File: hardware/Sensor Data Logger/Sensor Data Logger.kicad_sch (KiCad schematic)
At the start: 28 parts, among them J1 Conn_01x04_Male, J2 Conn_01x04_Male, J3 Conn_01x05_Male, J4 Conn_01x03_Male, SW1 SW_Push, SW2 SW_Push, SW3 SW_Push, U1 AMS1117-3.3, U2 ESP32-WROOM-32, U3 DS3231M

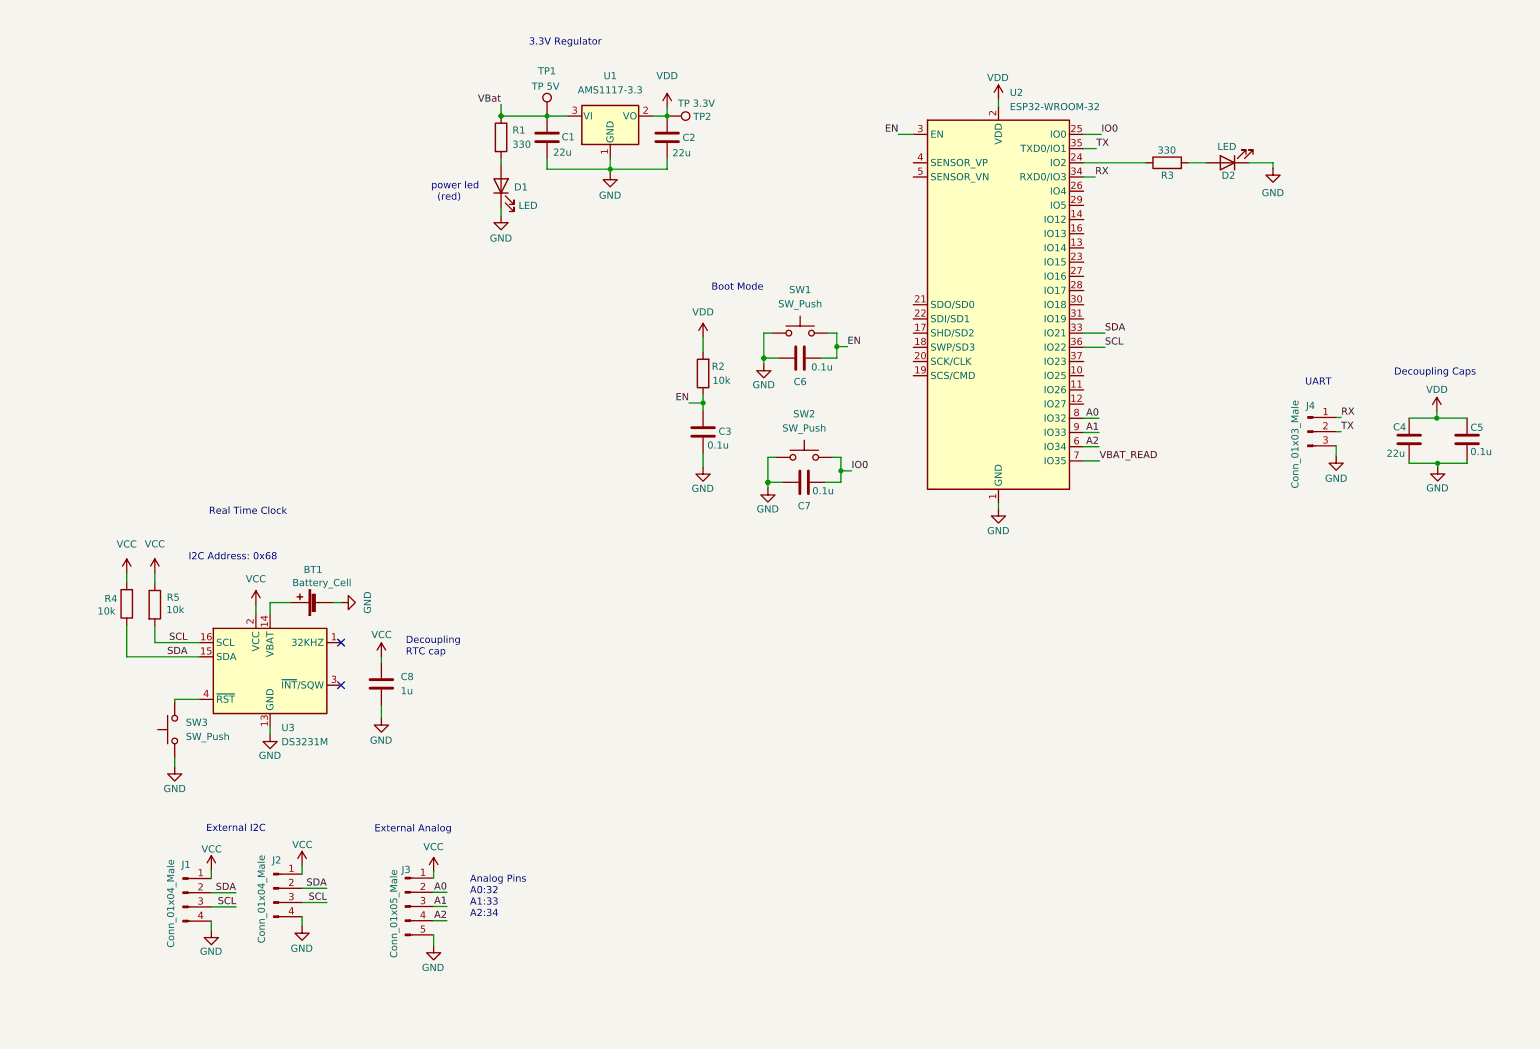
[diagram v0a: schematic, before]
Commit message: Latest schematic
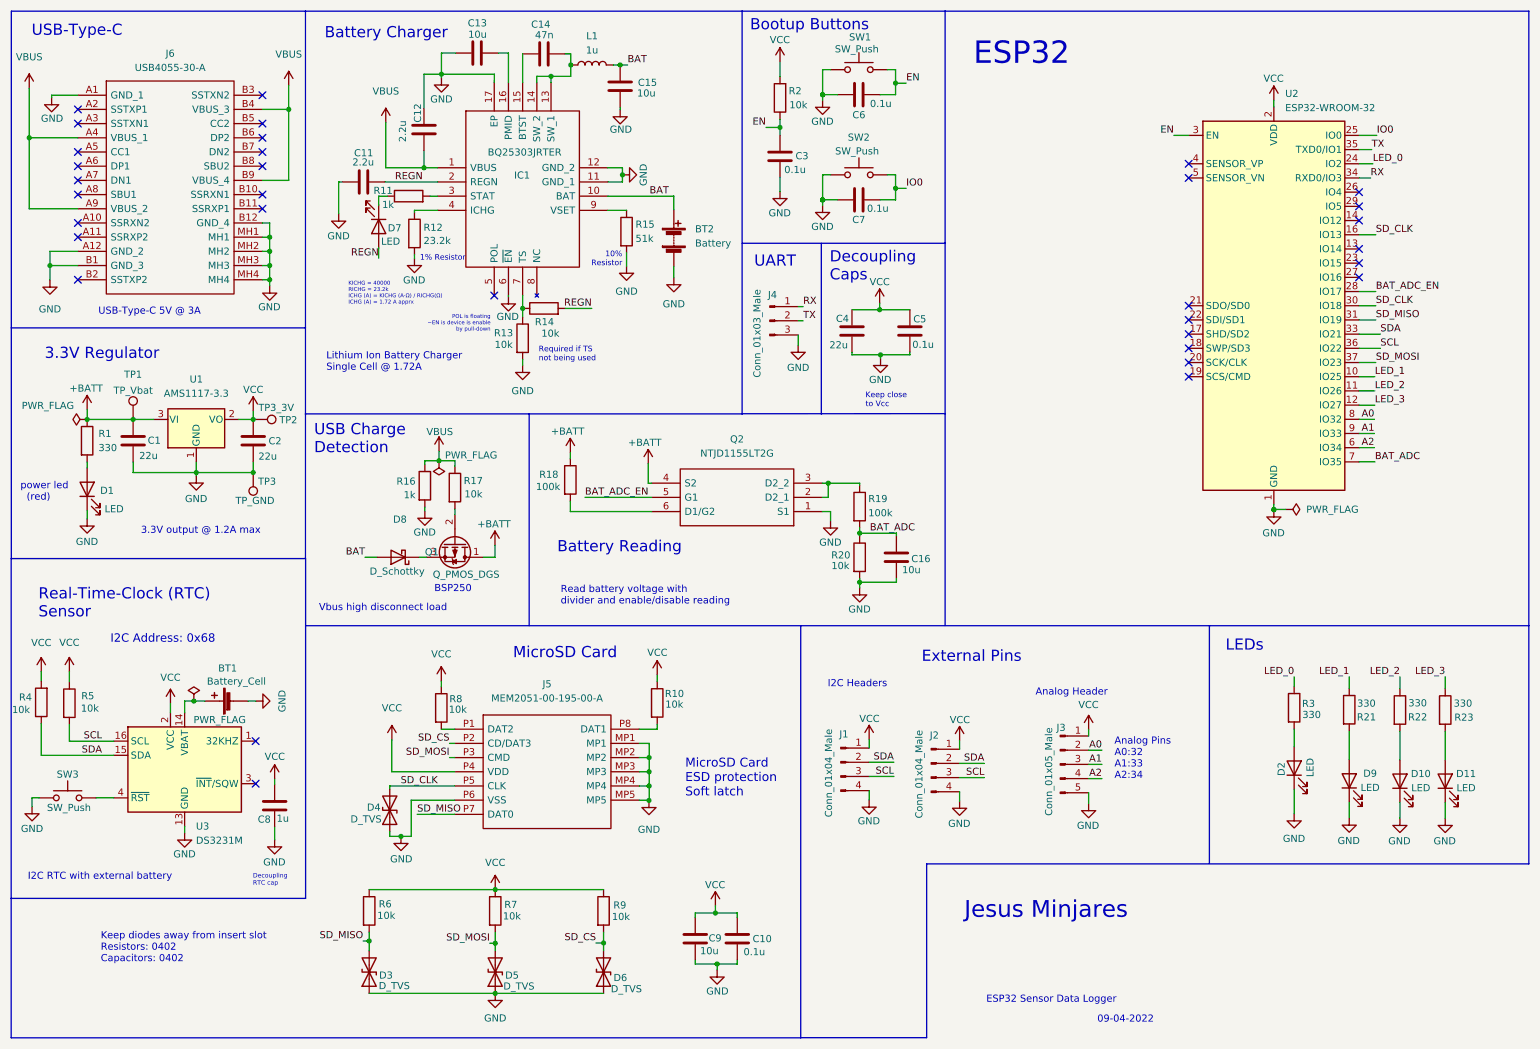
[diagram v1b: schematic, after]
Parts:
- added BT2: Battery, symbol Device:Battery
- added C10: 0.1u, symbol Device:C
- added C11, C12: 2.2u, symbol Device:C
- added C13, C15, C16, C9: 10u, symbol Device:C
- added C14: 47n, symbol Device:C
- added D10, D11, D7, D9: LED, symbol Device:LED
- added D3, D4, D5, D6: D_TVS, symbol Device:D_TVS
- added D8: D_Schottky, symbol Device:D_Schottky
- added IC1: BQ25303JRTER, Battery Charger:QFN50P300X300X80-17N-D, symbol Battery Charger:BQ25303JRTER
- added J5: MEM2051-00-195-00-A, Micro-SD Card:MEM20510019500A, symbol Micro-SD Card:MEM2051-00-195-00-A
- added J6: USB4055-30-A, USB-Type-C:USB405530A, symbol USB-Type-C:USB4055-30-A
- added L1: 1u, symbol Device:L
- added Q1: Q_PMOS_DGS, Package_TO_SOT_SMD:SOT-223-3_TabPin2, symbol Device:Q_PMOS_DGS
- added Q2: NTJD1155LT2G, SOT65P210X110-6N, symbol NTJD1155LT2G:NTJD1155LT2G
- added R10, R13, R14, R17, R20, R6, R7, R8, R9: 10k, symbol Device:R
- added R11, R16: 1k, symbol Device:R
- added R12: 23.2k, symbol Device:R
- added R15: 51k, symbol Device:R
- added R18, R19: 100k, symbol Device:R
- added R21, R22, R23: 330, symbol Device:R
- added TP3: TP_GND, symbol Connector:TestPoint
- TP1: value TP 5V -> TP_Vbat
- TP2: value TP 3.3V -> TP3_3V
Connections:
- net VDD is gone; now on net VCC: C2.1, C4.1, C5.1, R2.2, TP2.1, U1.2 (VO), U2.2 (VDD)
- net GND: now also BT2.2 (-), C10.2, C11.1, C12.1, C13.2, C15.2, C16.2, C9.2, D10.1 (K), D11.1 (K), D3.1 (A1), D4.1 (A1), D5.1 (A1), D6.1 (A1), D9.1 (K), IC1.11 (GND_1), IC1.12 (GND_2), IC1.17 (EP), IC1.6 (~{EN}), J5.P6 (VSS), J6.A1 (GND_1), J6.A12 (GND_2), J6.B1 (GND_3), J6.B12 (GND_4), J6.MH1, J6.MH2, J6.MH3, J6.MH4, Q2.1 (S1), R12.2, R13.2, R15.2, R16.2, R20.2, TP3.1
- net VCC: now also C10.1, C9.1, J5.P4 (VDD), R10.1, R6.1, R7.1, R8.1, R9.1
- net +BATT: now reaches C1.1, R1.1, TP1.1, U1.3 (VI)
- net +BATT: now also Q1.1 (D), Q2.4 (S2), R18.1
- net LED_1: now reaches U2.10 (IO25)
- net LED_1: now also R21.1
- net LED_2: now reaches U2.11 (IO26)
- net LED_2: now also R22.1
- net LED_3: now reaches U2.12 (IO27)
- net LED_3: now also R23.1
- net SD_CLK: now reaches U2.16 (IO13)
- net SD_CLK: now also U2.30 (IO18), D4.2 (A2), J5.P5 (CLK)
- net LED_0: now reaches R3.1, U2.24 (IO2)
- net BAT_ADC_EN: now reaches U2.28 (IO17)
- net BAT_ADC_EN: now also Q2.5 (G1)
- net SD_MISO: now reaches U2.31 (IO19)
- net SD_MISO: now also D3.2 (A2), J5.P7 (DAT0), R6.2
- net SD_MOSI: now reaches U2.37 (IO23)
- net SD_MOSI: now also D5.2 (A2), J5.P3 (CMD), R7.2
- net VBAT_READ renamed BAT_ADC
- net BAT_ADC: now also C16.1, R19.2, R20.1
- new net: IC1.7 (TS), R13.1, R14.1
- new net: Q1.2 (G), R17.2
- new net: C14.1, IC1.15 (BTST)
- new net: C14.2, IC1.13 (SW_1), IC1.14 (SW_2), L1.1
- new net: J5.P8 (DAT1), R10.2
- new net: D9.2 (A), R21.2
- new net: D10.2 (A), R22.2
- new net: D11.2 (A), R23.2
- new net: IC1.4 (ICHG), R12.1
- new net: C13.1, IC1.16 (PMID)
- new net: Q2.6 (D1/G2), R18.2
- new net: J5.MP1, J5.MP2, J5.MP3, J5.MP4, J5.MP5
- new net: J5.P1 (DAT2), R8.2
- new net: IC1.9 (VSET), R15.1
- new net: D8.1 (K), Q1.3 (S)
- new net: Q2.2 (D2_1), Q2.3 (D2_2), R19.1
- new net: IC1.3 (STAT), R11.2
- new net: D7.1 (K), R11.1
- new net BAT: BT2.1 (+), C15.1, D8.2 (A), IC1.10 (BAT), L1.2
- new net REGN: C11.2, D7.2 (A), IC1.2 (REGN), R14.2
- new net SD_CS: D6.2 (A2), J5.P2 (CD/DAT3), R9.2
- new net VBUS: C12.2, IC1.1 (VBUS), J6.A4 (VBUS_1), J6.A9 (VBUS_2), J6.B4 (VBUS_3), J6.B9 (VBUS_4), R16.1, R17.1
- no-connect marks 2 -> 33
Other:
- note added: "09-04-2022"
- note added: "1% Resistor"
- note added: "10% Resistor"
- note added: "3.3V output @ 1.2A max"
- note added: "Analog Header"
- note added: "BSP250"
- note added: "Battery Charger"
- note added: "Battery Reading"
- note added: "Bootup Buttons"
- note added: "ESP32"
- note added: "ESP32 Sensor Data Logger"
- note added: "External Pins"
- note added: "I2C Headers"
- note added: "I2C RTC with external battery"
- note added: "Jesus Minjares"
- note added: "KICHG = 40000 RICHG = 23.2k ICHG (A) = KICHG (A·Ω) / RICHG(Ω) ICHG (A) = 1.72 A apprx"
- note added: "Keep close to Vcc"
- note added: "Keep diodes away from insert slot Resistors: 0402 Capacitors: 0402"
- note added: "LEDs"
- note added: "Lithium Ion Battery Charger Single Cell @ 1.72A"
- note added: "MicroSD Card"
- note added: "MicroSD Card ESD protection Soft latch"
- note added: "POL is floating ~EN is device is enable by pull-down"
- note added: "Read battery voltage with divider and enable/disable reading"
- note added: "Real-Time-Clock (RTC) Sensor"
- note added: "Required if TS not being used"
- note added: "USB Charge Detection"
- note added: "USB-Type-C"
- note added: "USB-Type-C 5V @ 3A"
- note added: "Vbus high disconnect load"
- note removed: "Boot Mode"
- note removed: "External Analog"
- note removed: "External I2C"
- note removed: "Real Time Clock"
- moved on the sheet: BT1, C1, C2, C3, C4, C5, C6, C7, C8, D1, D2, J1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
